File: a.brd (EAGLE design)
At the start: 50 x 42.2 mm, 32 parts, among them CON1 PINHEAD_1X04-2.54, CON3 PINHEAD_1X07-2.54, SW1 TACT_SWITCH-1-1825910-4, SW2 TACT_SWITCH-1-1825910-4, X3 PINHEAD_1X06-2-MALE, X4 PINHEAD_2X03-PTH-2.54

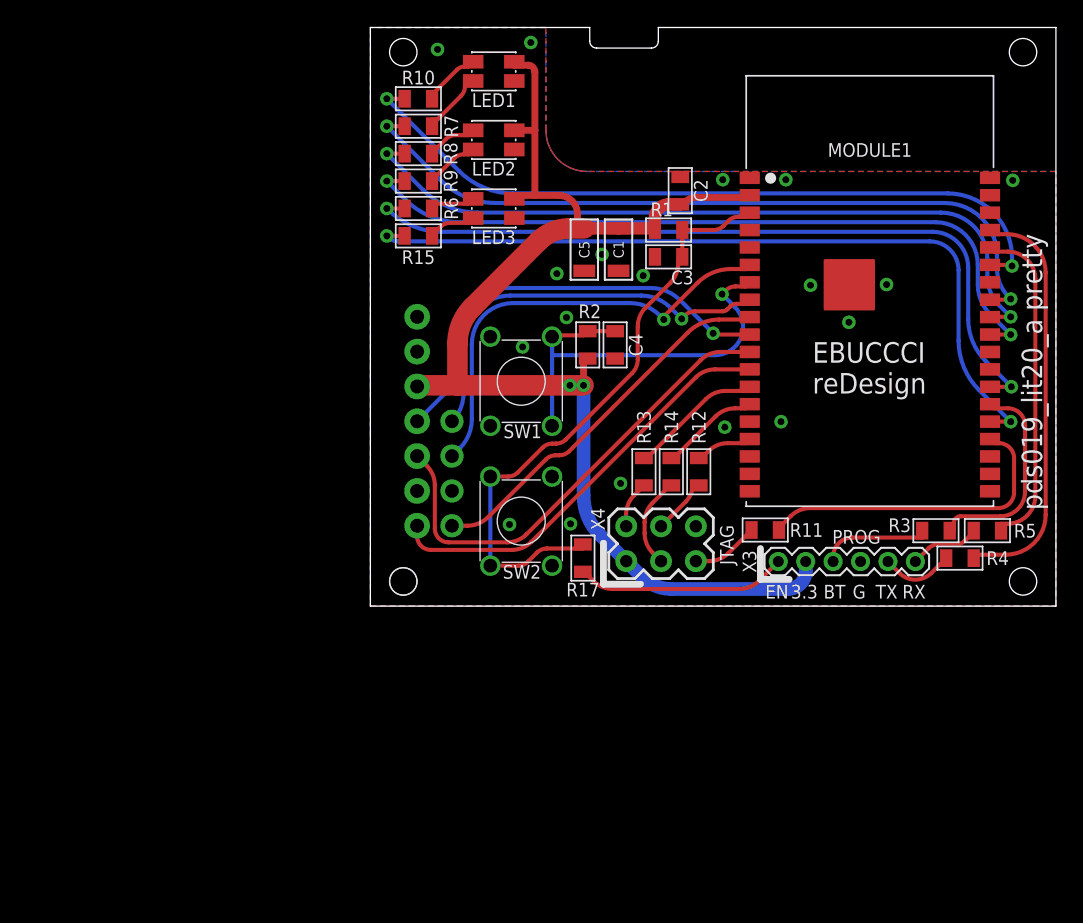
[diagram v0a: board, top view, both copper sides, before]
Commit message: A pcb updated
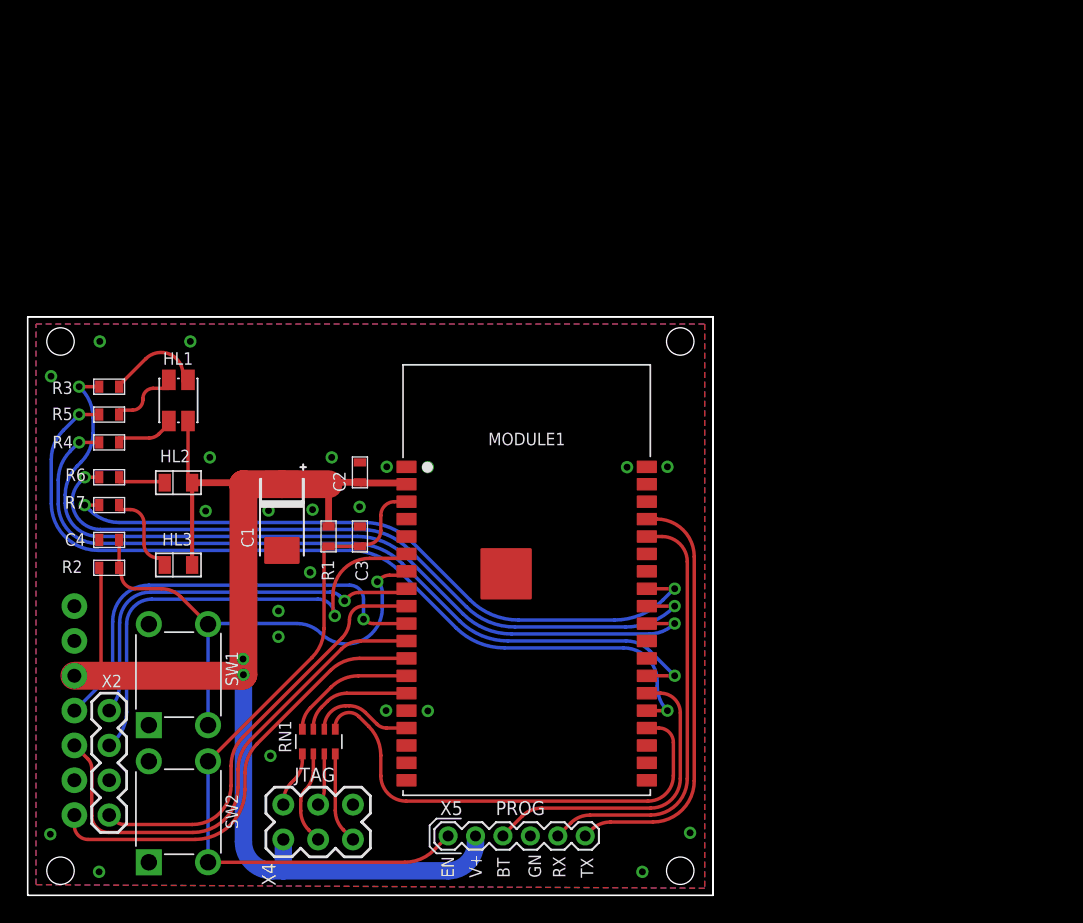
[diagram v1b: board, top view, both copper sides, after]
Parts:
- removed C5: 47u, rc:C1206
- removed CON1: PINHEAD_1X04-2.54, pinhead:1X04-PTH-2.54
- removed CON3: PINHEAD_1X07-2.54, pinhead:1X07-PTH-2.54
- removed LED1, LED2, LED3: LED_RGB-3528, rc:LED3528
- removed R10, R15, R8, R9: 1K, rc:R0805
- removed R11, R12, R13, R14, R17: 100R, rc:R0805
- removed U$1: (no value), ref:REF_A
- removed X3: PINHEAD_1X06-2-MALE, pinhead:1X06-PTH-2
- added HL1: LED_RGB-KAA-3528RGBS, rc:LED3528
- added HL2, HL3: LED-0805, rc:LED0805
- added RN1: 100R, rc:R_4X0603
- added U$2: (no value), pds019_lit:D3MG_PCB_UP
- added X1: PINHEAD_1X07-2.54, pinhead:1X07-PTH-2.54
- added X2: PINHEAD_1X04-2.54, pinhead:1X04-PTH-2.54
- added X5: PINHEAD_1X06-2-MALE, pinhead:1X06-PTH-2
- C1: value 47u -> 100u; device rc:C1206 -> rc:CTANT_TYPE_C
- C2, C3: value 0.1u -> 0.1; device rc:C0805 -> rc:C0603
- C4: device rc:C0805 -> rc:C0603
- R1, R2: device rc:R0805 -> rc:R0603
- R3: value 100R -> 3,3K*; device rc:R0805 -> rc:R0603
- R4: value 43R -> 8,2K*; device rc:R0805 -> rc:R0603
- R5: value 43R -> 12K*; device rc:R0805 -> rc:R0603
- R6, R7: value 1K -> 470R*; device rc:R0805 -> rc:R0603
- SW1: value TACT_SWITCH-1-1825910-4 -> TS6601-11; device mechanical:1-1825910-4 -> mechanical:SW4-6.0X6.0X5.0MM
- SW2: value TACT_SWITCH-1-1825910-4 -> TS6601-9,5; device mechanical:1-1825910-4 -> mechanical:SW4-6.0X6.0X5.0MM
- moved R5 64.6 mm to (-19.1, 14.0), turned to 0 degrees
- moved R4 62.6 mm to (-19.1, 11.9), turned to 0 degrees
- moved R3 61.2 mm to (-19.1, 16.0), turned to 0 degrees
- moved C4 39.5 mm to (-19.1, 4.83), turned to 0 degrees
- moved R2 38.5 mm to (-19.1, 2.79), turned to 180 degrees
- moved R7 35.7 mm to (-19.1, 7.37)
- moved R1 33.4 mm to (-3.05, 5.08), turned to 90 degrees
- moved SW1 32.9 mm to (-14.0, -5.00)
- moved SW2 32.8 mm to (-14.0, -15.0), turned to 90 degrees
- moved MODULE1 32.7 mm to (11.4, 1.90)
- moved X4 32.2 mm to (-3.81, -15.7)
- moved C1 31.4 mm to (-6.45, 6.48), turned to 270 degrees
- moved C2 31.1 mm to (-0.76, 9.75), turned to 270 degrees
- moved C3 30.4 mm to (-0.76, 5.08), turned to 270 degrees
- moved R6 29.9 mm to (-19.1, 9.40)
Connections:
- net G1LED renamed !LED_OUT
- removed net ESP_IO36: MODULE1.4
- removed net ESP_IO39: MODULE1.5
- removed net G2LED: MODULE1.29, R9.1
- removed net G3LED: MODULE1.24, R15.1
- removed net N$10: LED3.1, R6.2
- removed net N$11: LED3.4, R15.2
- removed net N$14: R14.1, X4.3
- removed net N$15: R11.1, X4.5
- removed net N$17: R17.2, X3.1
- removed net N$3: R5.2, X3.6
- removed net N$5: R3.2, X3.3
- removed net N$6: R12.2, X4.4
- removed net N$7: LED1.1, R10.2
- removed net N$9: LED2.4, R9.2
- removed net R1LED: MODULE1.33, R10.1
- removed net R2LED: MODULE1.30, R8.1
- removed net R3LED: MODULE1.26, R6.1
- new net !LED_B: MODULE1.24, R5.1
- new net !LED_G: MODULE1.26, R4.1
- new net !LED_IN: MODULE1.30, R6.1
- new net !LED_R: MODULE1.29, R3.1
- new net N$124: RN1.4, X4.5
- new net N$150: RN1.1, X4.2
- new net N$18: HL3.C, R7.2
- new net N$213: RN1.2, X4.3
- new net N$216: RN1.3, X4.4
- net ESP_BOOT: now also X5.3; no longer R3.1
- net ESP_EN: now also SW2.2, X5.1; no longer R17.1, SW2.4
- net ESP_IO25: now also X1.4; no longer CON3.4
- net ESP_IO26: now also X1.5; no longer CON3.5
- net ESP_IO27: now also X1.7; no longer CON3.7
- net ESP_IO32: now also X2.1; no longer CON1.1
- net ESP_IO33: now also X2.4; no longer CON1.4
- net ESP_IO34: now also X2.2; no longer CON1.2
- net ESP_IO35: now also C4.2, SW1.2; no longer C4.1, SW1.4
- net ESP_RXD0: now also X5.5; no longer R5.1
- net ESP_TXD0: now also X5.6; no longer R4.1
- net GND: now also C1.-, C2.1, C4.1, SW1.4, SW2.4, X1.2, X1.6, X2.3, X5.4; no longer C1.P$1, C2.2, C4.2, C5.P$1, CON1.3, CON3.2, CON3.6, SW1.2, SW2.2, X3.4
- net MTCK: now also RN1.6; no longer R12.1
- net MTDI: now also RN1.7; no longer R14.2
- net MTDO: now also RN1.5; no longer R11.2
- net MTMS: now also RN1.8; no longer R13.1
- net N$1: now also HL1.4, R5.2; no longer LED2.1, R8.2
- net N$2: now also HL1.3, R4.2; no longer R13.2, X4.2
- net N$4: now also HL1.1, R3.2; no longer R4.2, X3.5
- net N$8: now also HL2.C, R6.2; no longer LED1.4, R7.2
- net VDD_3V3: now also C1.+, C2.2, HL1.2, HL2.A, HL3.A, X1.3, X5.2; no longer C1.P$2, C2.1, C5.P$2, CON3.3, LED1.2, LED2.2, LED3.2, X3.2
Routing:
- net !LED_B: track 0.00 -> 61.3 mm, vias 0 -> 2
- net !LED_R: track 0.00 -> 60.6 mm, vias 0 -> 2
- net !LED_G: track 0.00 -> 57.8 mm, vias 0 -> 2
- net G3LED: track 57.8 -> 0.00 mm, vias 2 -> 0
- net R3LED: track 56.4 -> 0.00 mm, vias 2 -> 0
- net R2LED: track 54.2 -> 0.00 mm, vias 2 -> 0
- net G2LED: track 54.0 -> 0.00 mm, vias 2 -> 0
- net R1LED: track 53.6 -> 0.00 mm, vias 2 -> 0
- net !LED_IN: track 0.00 -> 51.8 mm, vias 0 -> 2
- net N$17: track 15.3 -> 0.00 mm
- net MTDO: track 23.1 -> 34.5 mm
- net ESP_EN: track 44.1 -> 52.5 mm
- net N$5: track 7.93 -> 0.00 mm
- net ESP_BOOT: track 15.0 -> 22.4 mm
- net N$213: track 0.00 -> 6.82 mm
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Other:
- outline, holes or cut-outs redrawn
- board text added: ">DRAWING_NAME"
- board text added: ">PLOT_DATE_TIME"
- board text added: "GN"
- board text added: "V+"
- board text removed: "2 layer PCB Copper thickness 35 uM Soldermask color blue PCB thickness 2 mm"
- board text removed: "3.3"
- board text removed: "EBUCCCI reDesign"
- board text removed: "G"
- board text removed: "pds019_lit20_a pretty"

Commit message: Import
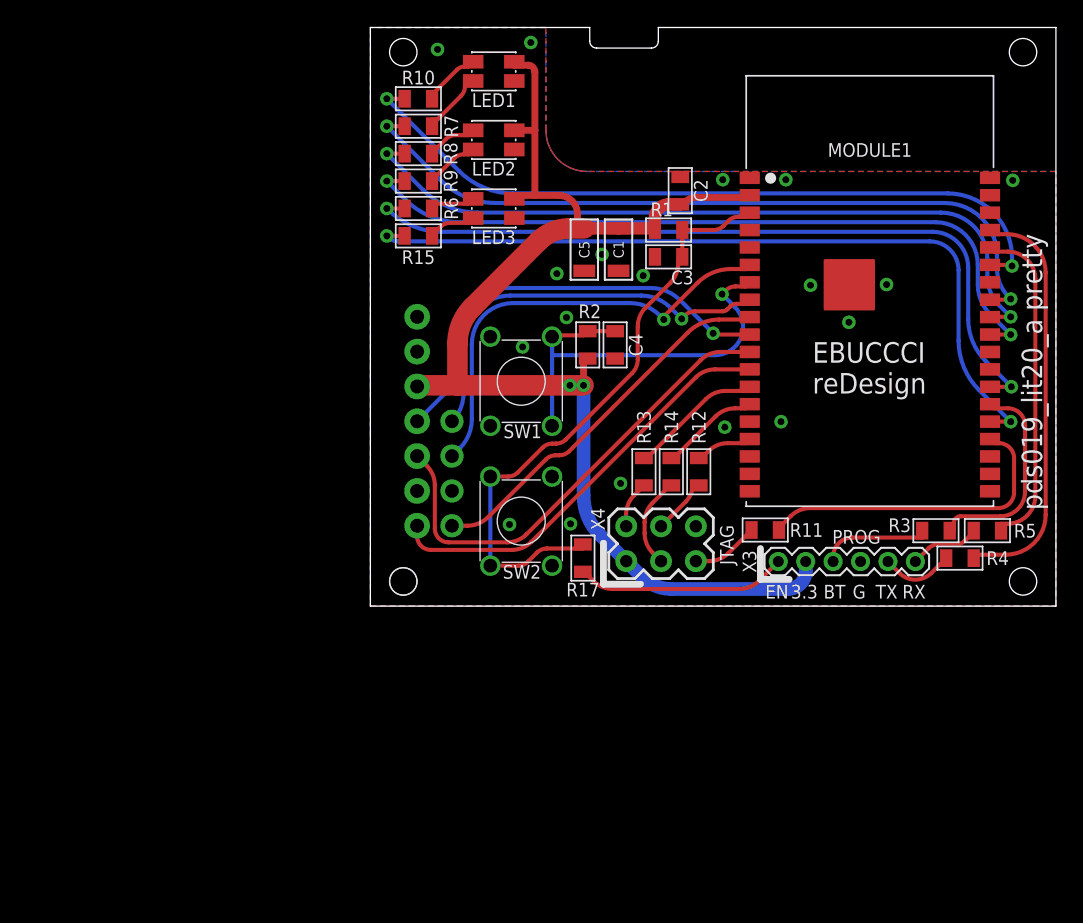
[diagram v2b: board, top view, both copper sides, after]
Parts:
- removed HL1: LED_RGB-KAA-3528RGBS, rc:LED3528
- removed HL2, HL3: LED-0805, rc:LED0805
- removed RN1: 100R, rc:R_4X0603
- removed U$2: (no value), pds019_lit:D3MG_PCB_UP
- removed X1: PINHEAD_1X07-2.54, pinhead:1X07-PTH-2.54
- removed X2: PINHEAD_1X04-2.54, pinhead:1X04-PTH-2.54
- removed X5: PINHEAD_1X06-2-MALE, pinhead:1X06-PTH-2
- added C5: 47u, rc:C1206
- added CON1: PINHEAD_1X04-2.54, pinhead:1X04-PTH-2.54
- added CON3: PINHEAD_1X07-2.54, pinhead:1X07-PTH-2.54
- added LED1, LED2, LED3: LED_RGB-3528, rc:LED3528
- added R10, R15, R8, R9: 1K, rc:R0805
- added R11, R12, R13, R14, R17: 100R, rc:R0805
- added U$1: (no value), ref:REF_A
- added X3: PINHEAD_1X06-2-MALE, pinhead:1X06-PTH-2
- C1: value 100u -> 47u; device rc:CTANT_TYPE_C -> rc:C1206
- C2, C3: value 0.1 -> 0.1u; device rc:C0603 -> rc:C0805
- C4: device rc:C0603 -> rc:C0805
- R1, R2: device rc:R0603 -> rc:R0805
- R3: value 3,3K* -> 100R; device rc:R0603 -> rc:R0805
- R4: value 8,2K* -> 43R; device rc:R0603 -> rc:R0805
- R5: value 12K* -> 43R; device rc:R0603 -> rc:R0805
- R6, R7: value 470R* -> 1K; device rc:R0603 -> rc:R0805
- SW1: value TS6601-11 -> TACT_SWITCH-1-1825910-4; device mechanical:SW4-6.0X6.0X5.0MM -> mechanical:1-1825910-4
- SW2: value TS6601-9,5 -> TACT_SWITCH-1-1825910-4; device mechanical:SW4-6.0X6.0X5.0MM -> mechanical:1-1825910-4
- moved R5 64.6 mm to (45.0, 5.50), turned to 180 degrees
- moved R4 62.6 mm to (43.0, 3.50), turned to 180 degrees
- moved R3 61.2 mm to (41.2, 5.50), turned to 180 degrees
- moved C4 39.5 mm to (17.9, 19.1), turned to 270 degrees
- moved R2 38.5 mm to (15.8, 19.1), turned to 270 degrees
- moved R7 35.7 mm to (3.50, 35.0)
- moved R1 33.4 mm to (21.8, 27.4), turned to 180 degrees
- moved SW1 32.9 mm to (11.0, 16.4)
- moved SW2 32.8 mm to (11.0, 6.20), turned to 270 degrees
- moved MODULE1 32.7 mm to (36.4, 23.0)
- moved X4 32.2 mm to (21.2, 4.55)
- moved C1 31.4 mm to (18.1, 26.0), turned to 90 degrees
- moved C2 31.1 mm to (22.6, 30.3), turned to 90 degrees
- moved C3 30.4 mm to (21.8, 25.5), turned to 0 degrees
- moved R6 29.9 mm to (3.50, 29.0)
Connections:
- net !LED_OUT renamed G1LED
- removed net !LED_B: MODULE1.24, R5.1
- removed net !LED_G: MODULE1.26, R4.1
- removed net !LED_IN: MODULE1.30, R6.1
- removed net !LED_R: MODULE1.29, R3.1
- removed net N$124: RN1.4, X4.5
- removed net N$150: RN1.1, X4.2
- removed net N$18: HL3.C, R7.2
- removed net N$213: RN1.2, X4.3
- removed net N$216: RN1.3, X4.4
- new net ESP_IO36: MODULE1.4
- new net ESP_IO39: MODULE1.5
- new net G2LED: MODULE1.29, R9.1
- new net G3LED: MODULE1.24, R15.1
- new net N$10: LED3.1, R6.2
- new net N$11: LED3.4, R15.2
- new net N$14: R14.1, X4.3
- new net N$15: R11.1, X4.5
- new net N$17: R17.2, X3.1
- new net N$3: R5.2, X3.6
- new net N$5: R3.2, X3.3
- new net N$6: R12.2, X4.4
- new net N$7: LED1.1, R10.2
- new net N$9: LED2.4, R9.2
- new net R1LED: MODULE1.33, R10.1
- new net R2LED: MODULE1.30, R8.1
- new net R3LED: MODULE1.26, R6.1
- net ESP_BOOT: now also R3.1; no longer X5.3
- net ESP_EN: now also R17.1, SW2.4; no longer SW2.2, X5.1
- net ESP_IO25: now also CON3.4; no longer X1.4
- net ESP_IO26: now also CON3.5; no longer X1.5
- net ESP_IO27: now also CON3.7; no longer X1.7
- net ESP_IO32: now also CON1.1; no longer X2.1
- net ESP_IO33: now also CON1.4; no longer X2.4
- net ESP_IO34: now also CON1.2; no longer X2.2
- net ESP_IO35: now also C4.1, SW1.4; no longer C4.2, SW1.2
- net ESP_RXD0: now also R5.1; no longer X5.5
- net ESP_TXD0: now also R4.1; no longer X5.6
- net GND: now also C1.P$1, C2.2, C4.2, C5.P$1, CON1.3, CON3.2, CON3.6, SW1.2, SW2.2, X3.4; no longer C1.-, C2.1, C4.1, SW1.4, SW2.4, X1.2, X1.6, X2.3, X5.4
- net MTCK: now also R12.1; no longer RN1.6
- net MTDI: now also R14.2; no longer RN1.7
- net MTDO: now also R11.2; no longer RN1.5
- net MTMS: now also R13.1; no longer RN1.8
- net N$1: now also LED2.1, R8.2; no longer HL1.4, R5.2
- net N$2: now also R13.2, X4.2; no longer HL1.3, R4.2
- net N$4: now also R4.2, X3.5; no longer HL1.1, R3.2
- net N$8: now also LED1.4, R7.2; no longer HL2.C, R6.2
- net VDD_3V3: now also C1.P$2, C2.1, C5.P$2, CON3.3, LED1.2, LED2.2, LED3.2, X3.2; no longer C1.+, C2.2, HL1.2, HL2.A, HL3.A, X1.3, X5.2
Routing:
- net !LED_B: track 61.3 -> 0.00 mm, vias 2 -> 0
- net !LED_R: track 60.6 -> 0.00 mm, vias 2 -> 0
- net !LED_G: track 57.8 -> 0.00 mm, vias 2 -> 0
- net G3LED: track 0.00 -> 57.8 mm, vias 0 -> 2
- net R3LED: track 0.00 -> 56.4 mm, vias 0 -> 2
- net R2LED: track 0.00 -> 54.2 mm, vias 0 -> 2
- net G2LED: track 0.00 -> 54.0 mm, vias 0 -> 2
- net R1LED: track 0.00 -> 53.6 mm, vias 0 -> 2
- net !LED_IN: track 51.8 -> 0.00 mm, vias 2 -> 0
- net N$17: track 0.00 -> 15.3 mm
- net MTDO: track 34.5 -> 23.1 mm
- net ESP_EN: track 52.5 -> 44.1 mm
- net N$5: track 0.00 -> 7.93 mm
- net ESP_BOOT: track 22.4 -> 15.0 mm
- net N$213: track 6.82 -> 0.00 mm
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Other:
- outline, holes or cut-outs redrawn
- board text added: "2 layer PCB Copper thickness 35 uM Soldermask color blue PCB thickness 2 mm"
- board text added: "3.3"
- board text added: "EBUCCCI reDesign"
- board text added: "G"
- board text added: "pds019_lit20_a pretty"
- board text removed: ">DRAWING_NAME"
- board text removed: ">PLOT_DATE_TIME"
- board text removed: "GN"
- board text removed: "V+"
